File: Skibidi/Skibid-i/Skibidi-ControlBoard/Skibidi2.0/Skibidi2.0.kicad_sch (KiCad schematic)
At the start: 72 parts, among them IC1 TEENSY_4.1, J1 Conn_02x05_Odd_Even, J10 Screw_Terminal_01x03, J12 Screw_Terminal_01x03, J13 P78E05-1000, J15 Conn_01x03_Pin, J17 Conn_01x08_Pin, J19 12V, J2 Screw_Terminal_01x03, J20 Screw_Terminal_01x03, J3 Screw_Terminal_01x03, J4 Screw_Terminal_01x03, J5 Screw_Terminal_01x03, J6 Screw_Terminal_01x03, J7 Screw_Terminal_01x03, J8 Screw_Terminal_01x03, J9 Screw_Terminal_01x03, Q1 WL-OCPT_SERIES_357, Q2 WL-OCPT_SERIES_357, Q3 WL-OCPT_SERIES_357, Q4 WL-OCPT_SERIES_357, Q5 WL-OCPT_SERIES_357, Q6 WL-OCPT_SERIES_357, Q7 WL-OCPT_SERIES_357, SW1 SW_Nidec_CAS-120A1, SW2 210-4MS

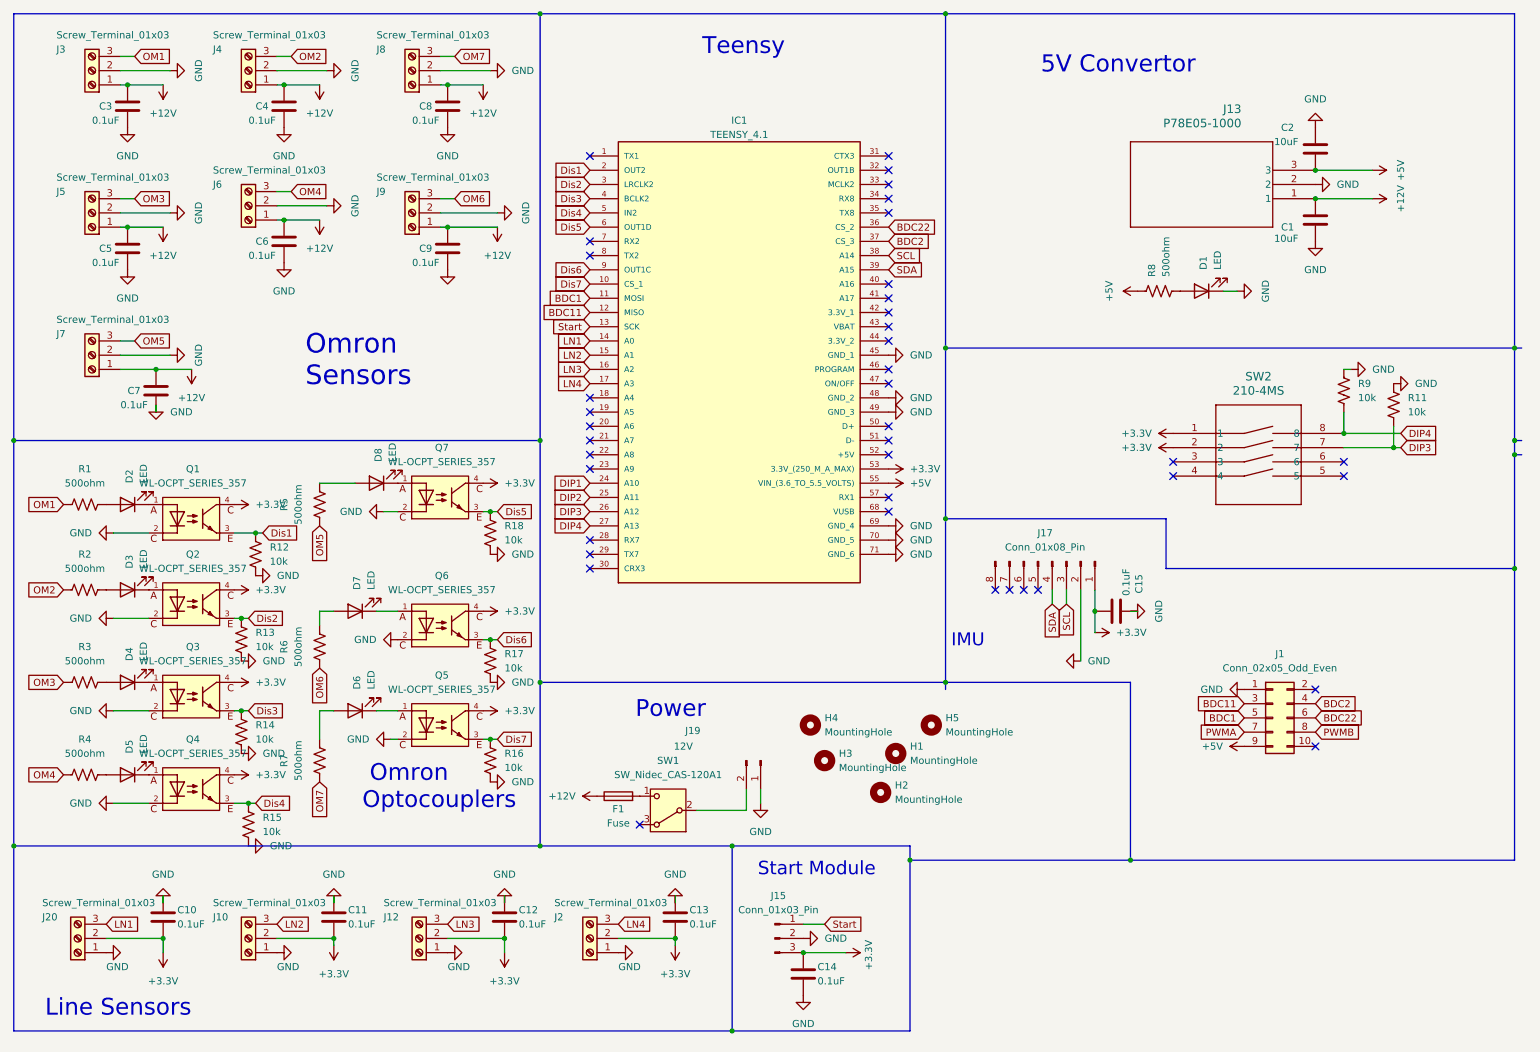
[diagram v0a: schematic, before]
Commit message: made a whole new pcb for voltage divider
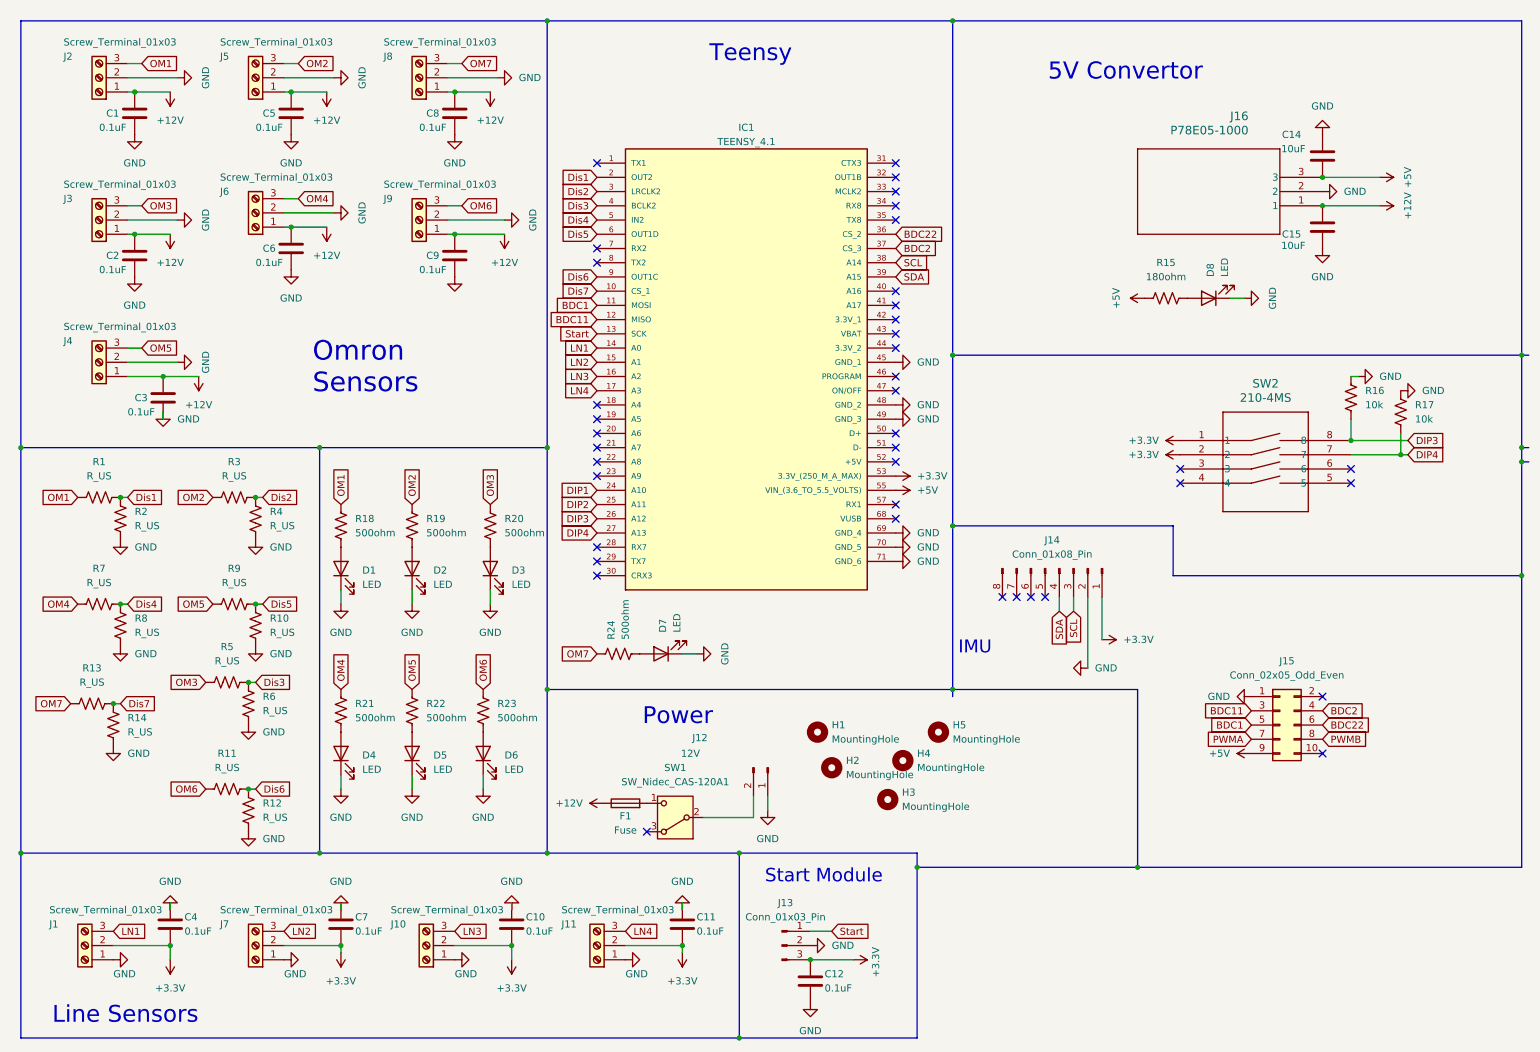
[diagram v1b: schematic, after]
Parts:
- removed C13: 0.1uF, Capacitor_SMD:C_0805_2012Metric, symbol Device:C
- removed J1: Conn_02x05_Odd_Even, Connector_PinSocket_2.54mm:PinSocket_2x05_P2.54mm_Vertical, symbol Connector_Generic:Conn_02x05_Odd_Even
- removed J12: Screw_Terminal_01x03, TerminalBlock:TerminalBlock_Xinya_XY308-2.54-3P_1x03_P2.54mm_Horizontal, symbol Connector:Screw_Terminal_01x03
- removed J13: P78E05-1000, askibidi:5vregulator, symbol convertor:P78E05-1000
- removed J15: Conn_01x03_Pin, Connector_PinHeader_2.54mm:PinHeader_1x03_P2.54mm_Vertical, symbol Connector:Conn_01x03_Pin
- removed J17: Conn_01x08_Pin, Connector_PinHeader_2.54mm:PinHeader_1x08_P2.54mm_Vertical, symbol Connector:Conn_01x08_Pin
- removed J19: 12V, Connector_AMASS:AMASS_XT30U-F_1x02_P5.0mm_Vertical, symbol Connector:Conn_01x02_Pin
- removed J20: Screw_Terminal_01x03, askibidi:Screwterimanl3, symbol Connector:Screw_Terminal_01x03
- removed Q1, Q2, Q3, Q4, Q5, Q6, Q7: WL-OCPT_SERIES_357, askibidi:optopt, symbol Optocouipler1]:WL-OCPT_SERIES_357
- added J1, J11: Screw_Terminal_01x03, TerminalBlock:TerminalBlock_Xinya_XY308-2.54-3P_1x03_P2.54mm_Horizontal, symbol Connector:Screw_Terminal_01x03
- added J12: 12V, Connector_AMASS:AMASS_XT30U-F_1x02_P5.0mm_Vertical, symbol Connector:Conn_01x02_Pin
- added J13: Conn_01x03_Pin, Connector_PinHeader_2.54mm:PinHeader_1x03_P2.54mm_Vertical, symbol Connector:Conn_01x03_Pin
- added J14: Conn_01x08_Pin, Connector_PinHeader_2.54mm:PinHeader_1x08_P2.54mm_Vertical, symbol Connector:Conn_01x08_Pin
- added J15: Conn_02x05_Odd_Even, Connector_PinSocket_2.54mm:PinSocket_2x05_P2.54mm_Vertical, symbol Connector_Generic:Conn_02x05_Odd_Even
- added J16: P78E05-1000, askibidi:5vregulator, symbol convertor:P78E05-1000
- added R10: R_US, Resistor_SMD:R_1206_3216Metric, symbol Device:R_US
- added R19, R20, R21, R22, R23, R24: 500ohm, Resistor_SMD:R_1206_3216Metric, symbol Device:R_US
- C1, C2: value 10uF -> 0.1uF
- C14, C15: value 0.1uF -> 10uF
- R1, R2, R3, R4, R5, R6, R7, R8: value 500ohm -> R_US; footprint Resistor_SMD:R_0805_2012Metric -> Resistor_SMD:R_1206_3216Metric
- R11, R9: value 10k -> R_US; footprint Capacitor_SMD:C_1206_3216Metric -> Resistor_SMD:R_1206_3216Metric
- R12, R13, R14: value 10k -> R_US; footprint Resistor_SMD:R_0805_2012Metric -> Resistor_SMD:R_1206_3216Metric
- R15: value 10k -> 180ohm
- R16, R17: footprint Resistor_SMD:R_0805_2012Metric -> Capacitor_SMD:C_1206_3216Metric
- R18: value 10k -> 500ohm; footprint Resistor_SMD:R_0805_2012Metric -> Resistor_SMD:R_1206_3216Metric
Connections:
- net +12V: now also C1.1, C15.2, C2.1, J2.1 (Pin_1), J16.1; no longer C1.2, C4.1, C7.1, J7.1 (Pin_1)
- net +3.3V: now also C12.1, C4.2, C7.2, J7.2 (Pin_2), J1.2 (Pin_2), J11.2 (Pin_2), J13.3 (Pin_3), J14.1 (Pin_1); no longer C12.2, C14.1, C15.2, J2.2 (Pin_2)
- net +5V: now also C14.1, R15.2, J15.9 (Pin_9), J16.3; no longer C2.1, R8.2
- net BDC1: now also J15.5 (Pin_5)
- net BDC11: now also J15.3 (Pin_3)
- net BDC2: now also J15.4 (Pin_4)
- net BDC22: now also J15.6 (Pin_6)
- net DIP3: now also R16.2, SW2.8; no longer R11.1, SW2.7
- net DIP4: now also R17.1, SW2.7; no longer R9.2, SW2.8
- net Dis1: now also R1.2, R2.2; no longer R12.2
- net Dis2: now also R3.2, R4.2; no longer R13.2
- net Dis3: now also R5.2, R6.2; no longer R14.2
- net Dis4: now also R7.2, R8.2; no longer R15.2
- net Dis5: now also R9.2, R10.2; no longer R18.2
- net Dis6: now also R11.2, R12.2; no longer R17.2
- net Dis7: now also R13.2, R14.2; no longer R16.2
- net GND: now also C1.2, C12.2, C4.1, C7.1, D2.1 (K), D3.1 (K), D4.1 (K), D5.1 (K), D6.1 (K), D7.1 (K), D8.1 (K), J2.2 (Pin_2), J7.1 (Pin_1), R17.2, R2.1, R4.1, R6.1, R8.1, J1.1 (Pin_1), J11.1 (Pin_1), J12.1 (Pin_1), J13.2 (Pin_2), J14.2 (Pin_2), J15.1 (Pin_1), J16.2, R10.1; no longer C1.1, C12.1, C4.2, C7.2, J2.1 (Pin_1), J7.2 (Pin_2), R11.2, R13.1, R15.1, R17.1, R18.1, R9.1
- net LN1: now also J1.3 (Pin_3)
- net LN2: now also J7.3 (Pin_3); no longer J10.3 (Pin_3)
- net LN3: now also J10.3 (Pin_3)
- net LN4: now also J11.3 (Pin_3); no longer J2.3 (Pin_3)
- net OM1: now also J2.3 (Pin_3), R18.2; no longer J3.3 (Pin_3)
- net OM2: now also J5.3 (Pin_3), R3.1, R19.2; no longer J4.3 (Pin_3), R2.1
- net OM3: now also J3.3 (Pin_3), R5.1, R20.2; no longer J5.3 (Pin_3), R3.1
- net OM4: now also R7.1, R21.2; no longer R4.1
- net OM5: now also J4.3 (Pin_3), R9.1, R22.2; no longer J7.3 (Pin_3), R5.1
- net OM6: now also R11.1, R23.2; no longer R6.1
- net OM7: now also R13.1, R24.2; no longer R7.1
- net PWMA: now also J15.7 (Pin_7)
- net PWMB: now also J15.8 (Pin_8)
- net SCL: now also J14.3 (Pin_3)
- net SDA: now also J14.4 (Pin_4)
- net Start: now also J13.1 (Pin_1)
- net at D2.2 (A): now also R19.1; no longer R1.2
- net at D5.2 (A): now also R22.1; no longer R4.2
- net at D8.2 (A): now also R15.1; no longer R5.2
- net at D4.2 (A): now also R21.1; no longer R3.2
- net at D6.2 (A): now also R23.1; no longer R7.2
- net at SW1.2 (B): now also J12.2 (Pin_2)
- net at D1.2 (A): now also R18.1; no longer R8.1
- net at D3.2 (A): now also R20.1; no longer R2.2
- net at D7.2 (A): now also R24.1; no longer R6.2
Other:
- note removed: "Omron Optocouplers"

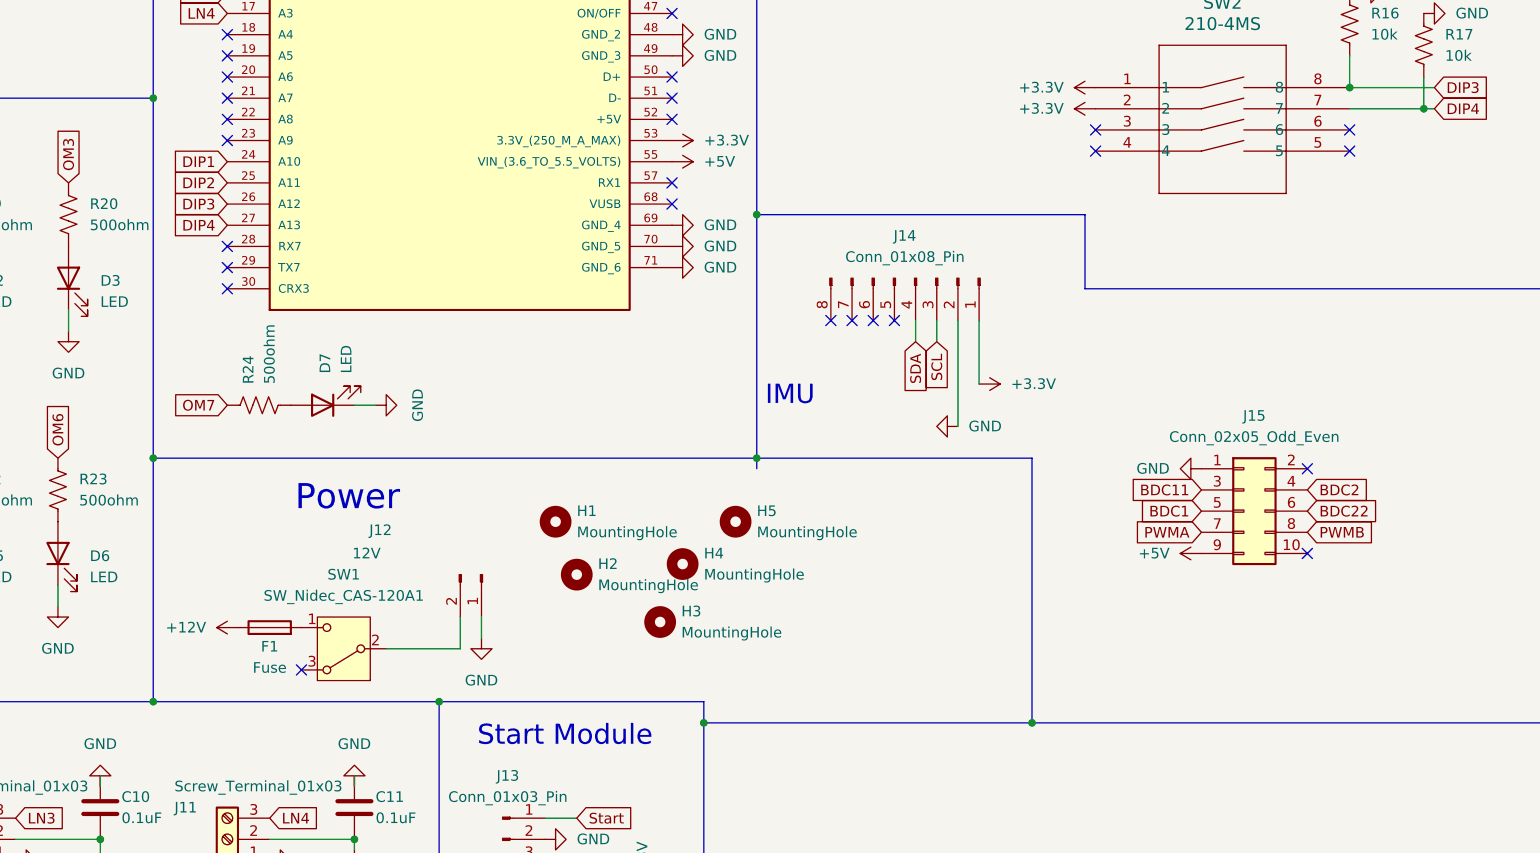
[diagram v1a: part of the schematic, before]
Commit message: skibidi 2.0 done
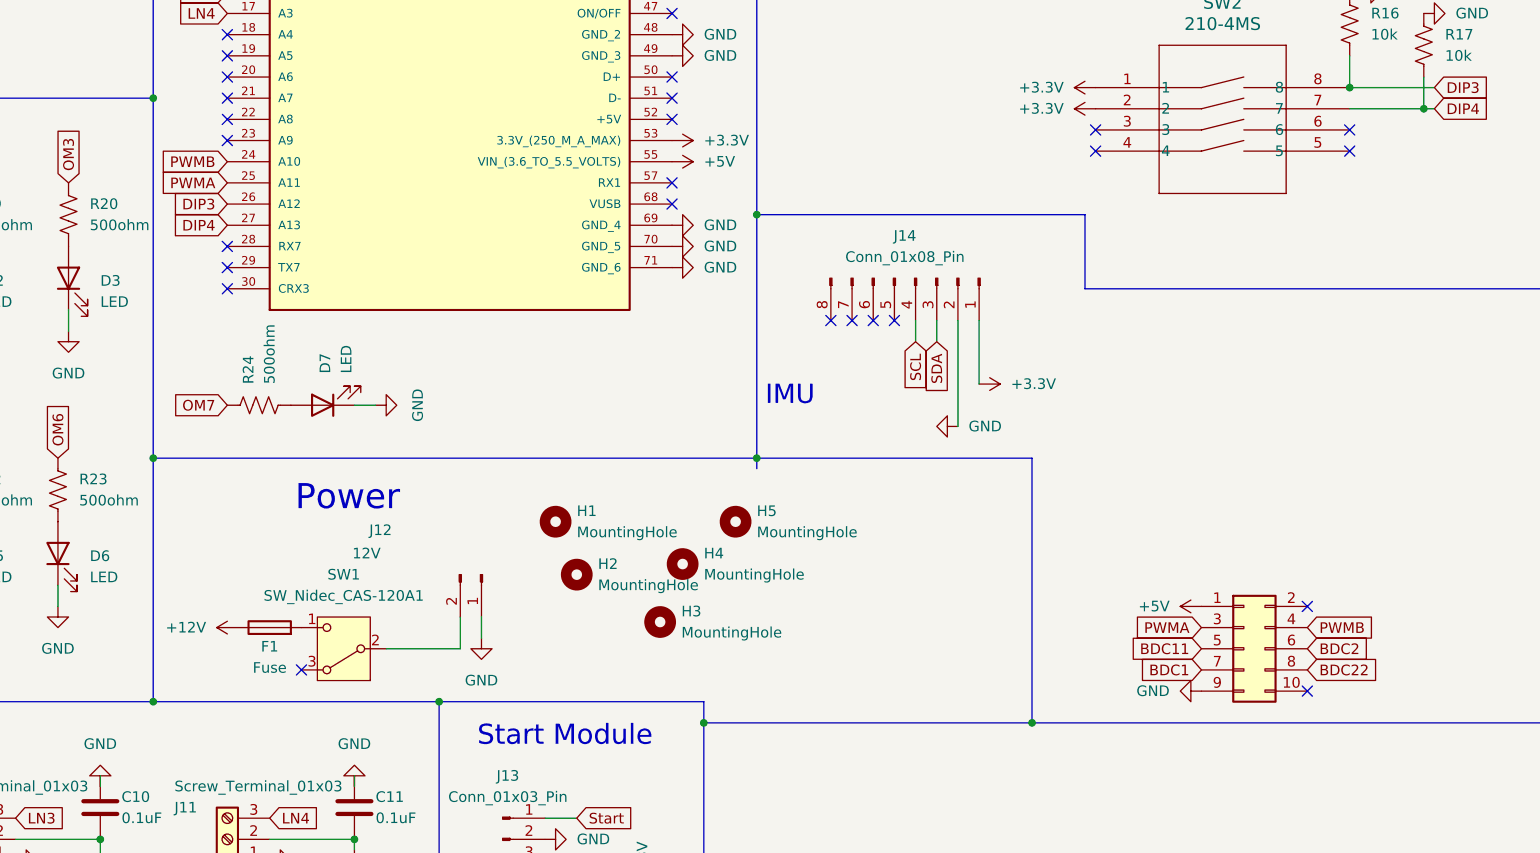
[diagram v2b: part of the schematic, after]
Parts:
- removed J15: Conn_02x05_Odd_Even, Connector_PinSocket_2.54mm:PinSocket_2x05_P2.54mm_Vertical, symbol Connector_Generic:Conn_02x05_Odd_Even
- added J17: Conn_02x05_Odd_Even, Connector_PinSocket_2.54mm:PinSocket_2x05_P2.54mm_Vertical, symbol Connector_Generic:Conn_02x05_Odd_Even
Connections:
- net DIP1 is gone; now on net PWMB: IC1.24 (A10)
- net DIP2 is gone; now on net PWMA: IC1.25 (A11)
- net +5V: now also J17.1 (Pin_1)
- net BDC1: now also J17.7 (Pin_7)
- net BDC11: now also J17.5 (Pin_5)
- net BDC2: now also J17.6 (Pin_6)
- net BDC22: now also J17.8 (Pin_8)
- net GND: now also J17.9 (Pin_9)
- net PWMA: now also J17.3 (Pin_3)
- net PWMB: now also J17.4 (Pin_4)
- net SCL: now also J14.4 (Pin_4); no longer J14.3 (Pin_3)
- net SDA: now also J14.3 (Pin_3); no longer J14.4 (Pin_4)
